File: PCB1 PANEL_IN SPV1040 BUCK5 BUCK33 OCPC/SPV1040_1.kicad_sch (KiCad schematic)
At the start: 14 parts, among them J2 SOLAR, U2 SPV1040TTR

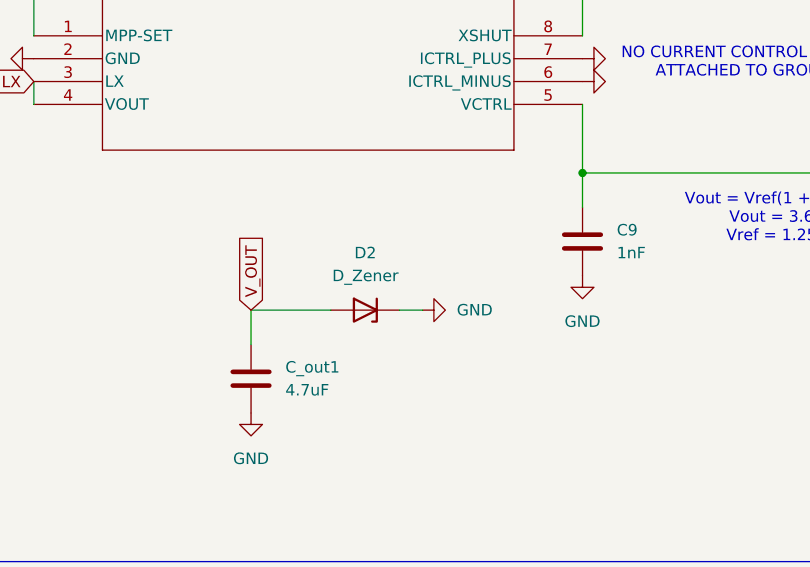
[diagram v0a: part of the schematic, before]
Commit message: w
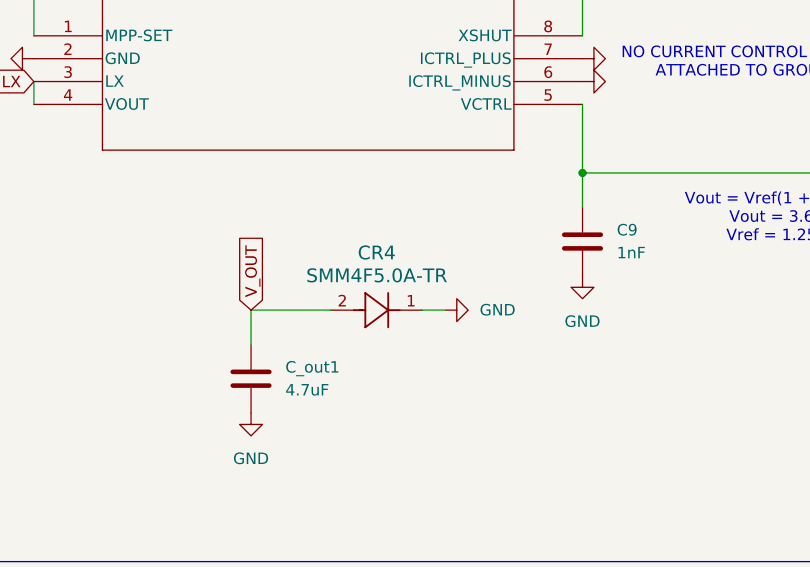
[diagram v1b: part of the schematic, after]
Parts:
- removed D2: D_Zener, Diode_SMD:D_1210_3225Metric, symbol Device:D_Zener
- added CR4: SMM4F5.0A-TR, CR_F5.0A-TR_STM, symbol SMM4F5:SMM4F5.0A-TR
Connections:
- net GND: now also CR4.1
- net PANEL1_OUT: now also CR4.2
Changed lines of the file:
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@@
-	(wire
-		(pts
-			(xy 105.41 95.25) (xy 107.95 95.25)
-		)
-		(stroke
-			(width 0)
-			(type default)
-		)
-	)
 	(wire
 		(pts
@@
 		(pts
 			(xy 167.64 27.94) (xy 213.36 27.94)
+		)
+		(stroke
+			(width 0)
+			(type default)
+		)
+	)
+	(wire
+		(pts
+			(xy 110.49 95.25) (xy 107.95 95.25)
 		)
 		(stroke
@@
 	)
 	(symbol
-		(lib_id "Device:D_Zener")
-		(at 101.6 95.25 180)
-		(unit 1)
-		(exclude_from_sim no)
-		(in_bom yes)
-		(on_board yes)
-		(dnp no)
-		(fields_autoplaced yes)
-		(property "Reference" "D2"
-			(at 101.6 88.9 0)
-			(effects
-				(font
-					(size 1.27 1.27)
-				)
-			)
-		)
-		(property "Value" "D_Zener"
-			(at 101.6 91.44 0)
-			(effects
-				(font
-					(size 1.27 1.27)
-				)
-			)
-		)
-		(property "Footprint" "Diode_SMD:D_1210_3225Metric"
-			(at 101.6 95.25 0)
-			(effects
-				(font
-					(size 1.27 1.27)
-				)
-				(hide yes)
-			)
-		)
-		(property "Datasheet" "~"
-			(at 101.6 95.25 0)
-			(effects
-				(font
-					(size 1.27 1.27)
-				)
-				(hide yes)
-			)
-		)
-		(property "Description" "Zener diode"
-			(at 101.6 95.25 0)
-			(effects
-				(font
-					(size 1.27 1.27)
-				)
-				(hide yes)
-			)
-		)
-		(pin "2"
-		)
-		(pin "1"
-		)
-		(instances
-			(project "PCB1 PANEL_IN SPV1040 BUCK5 BUCK33 OCPC"
-				(path "/494c9d9f-6b33-4248-a813-27ffaaa929bd/e53a10ab-2cc0-41d1-82dc-2525f18f01bb"
-					(reference "D2")
-					(unit 1)
-				)
-			)
-		)
-	)
-	(symbol
 		(lib_id "Device:C")
 		(at 125.73 87.63 0)
@@
 	)
 	(symbol
+		(lib_id "SMM4F5:SMM4F5.0A-TR")
+		(at 97.79 95.25 0)
+		(unit 1)
+		(exclude_from_sim no)
+		(in_bom yes)
+		(on_board yes)
+		(dnp no)
+		(fields_autoplaced yes)
+		(property "Reference" "CR4"
+			(at 102.87 88.9 0)
+			(effects
+				(font
+					(size 1.524 1.524)
+				)
+			)
+		)
+		(property "Value" "SMM4F5.0A-TR"
+			(at 102.87 91.44 0)
+			(effects
+				(font
+					(size 1.524 1.524)
+				)
+			)
+		)
+		(property "Footprint" "CR_F5.0A-TR_STM"
+			(at 97.79 95.25 0)
+			(effects
+				(font
+					(size 1.27 1.27)
+					(italic yes)
+				)
+				(hide yes)
+			)
+		)
+		(property "Datasheet" "SMM4F5.0A-TR"
+			(at 97.79 95.25 0)
+			(effects
+				(font
+					(size 1.27 1.27)
+					(italic yes)
+				)
+				(hide yes)
+			)
+		)
+		(property "Description" ""
+			(at 97.79 95.25 0)
+			(effects
+				(font
+					(size 1.27 1.27)
+				)
+				(hide yes)
+			)
+		)
+		(pin "1"
+		)
+		(pin "2"
+		)
+		(instances
+			(project "PCB1 PANEL_IN SPV1040 BUCK5 BUCK33 OCPC"
+				(path "/494c9d9f-6b33-4248-a813-27ffaaa929bd/e53a10ab-2cc0-41d1-82dc-2525f18f01bb"
+					(reference "CR4")
+					(unit 1)
+				)
+			)
+		)
+	)
+	(symbol
 		(lib_id "power:GND")
-		(at 107.95 95.25 90)
+		(at 110.49 95.25 90)
 		(unit 1)
 		(exclude_from_sim no)
@@
 		(fields_autoplaced yes)
 		(property "Reference" "#PWR011"
-			(at 114.3 95.25 0)
+			(at 116.84 95.25 0)
 			(effects
 				(font
@@
 		)
 		(property "Value" "GND"
-			(at 111.76 95.2499 90)
+			(at 114.3 95.2499 90)
 			(effects
 				(font
@@
 		)
 		(property "Footprint" ""
-			(at 107.95 95.25 0)
+			(at 110.49 95.25 0)
 			(effects
 				(font
@@
 		)
 		(property "Datasheet" ""
-			(at 107.95 95.25 0)
+			(at 110.49 95.25 0)
 			(effects
 				(font
@@
 		)
 		(property "Description" "Power symbol creates a global label with name \"GND\" , ground"
-			(at 107.95 95.25 0)
-			(effects
-				(font
+			(at 110.49 95.25 0)
+			(effects
+				(font
